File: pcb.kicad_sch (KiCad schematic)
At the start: 16 parts, among them IC1 BQ25606RGER, J1 PTHF-126-02-GF-Q-368, J1 Screw_Terminal_01x05, J2 Screw_Terminal_01x05, J3 Conn_01x01_Male

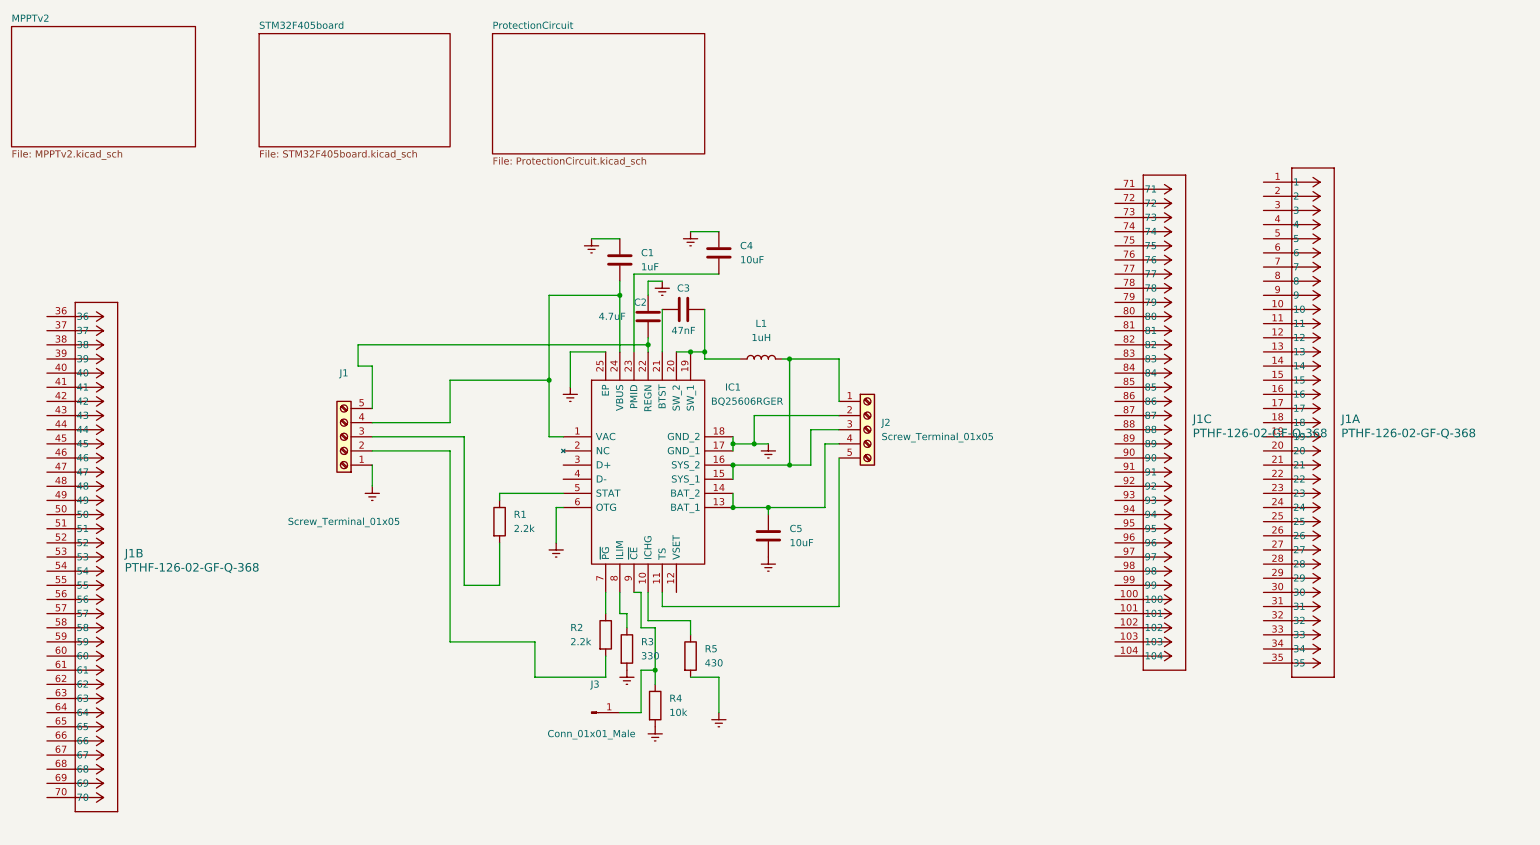
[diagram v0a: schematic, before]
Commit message: Major
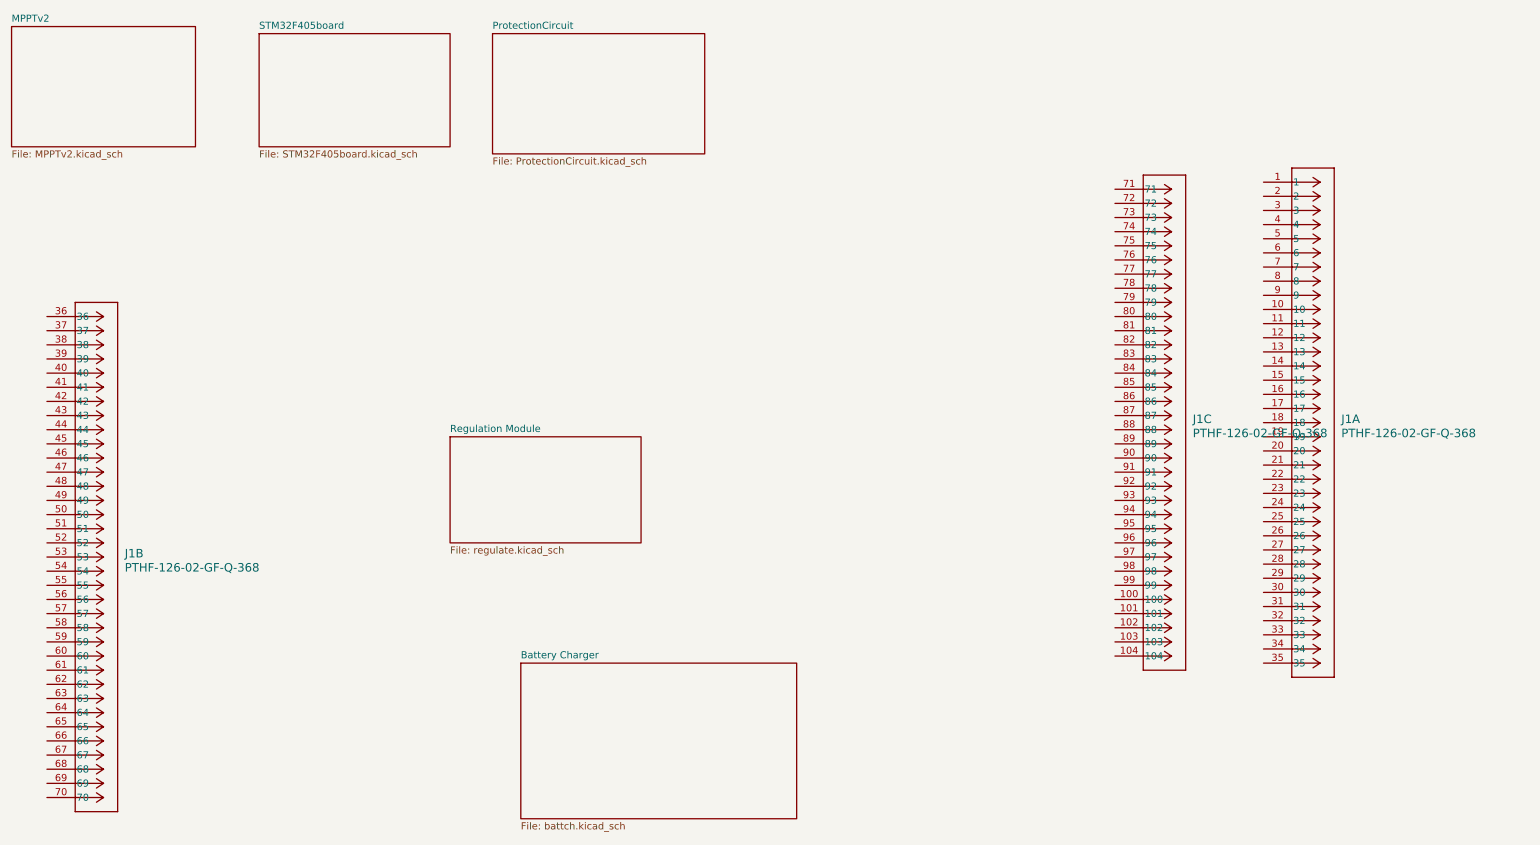
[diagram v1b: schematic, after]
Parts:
- removed C1: 1uF, 1uF cap:C1206, symbol Device:C
- removed C2: 4.7uF, cap 4.7uf:C1210, symbol Device:C
- removed C3: 47nF, 47nF:C1005_Commercial, symbol Device:C
- removed C4, C5: 10uF, 10uF MLCC:CAPC2012X94N, symbol Device:C
- removed IC1: BQ25606RGER, QFN50P400X400X100-25N-D, symbol BQ25606RGER:BQ25606RGER
- removed J1, J2: Screw_Terminal_01x05, TerminalBlock_MetzConnect:TerminalBlock_MetzConnect_Type059_RT06305HBWC_1x05_P3.50mm_Horizontal, symbol Connector:Screw_Terminal_01x05
- removed J3: Conn_01x01_Male, Connector_PinHeader_1.00mm:PinHeader_1x01_P1.00mm_Vertical, symbol Connector:Conn_01x01_Male
- removed L1: 1uH, 1uH indc:IHHP0805ZHER1R0M01, symbol Device:L
- removed R1, R2: 2.2k, 2.2k rst:RESC2012X65N, symbol Device:R
- removed R3: 330, rst 330:H2C_H2R, symbol Device:R
- removed R4: 10k, 10k rst:ERA8KEB1004V, symbol Device:R
- removed R5: 430, rst 430:ERJH3, symbol Device:R
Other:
- added sheet Battery Charger (battch.kicad_sch)
- added sheet Regulation Module (regulate.kicad_sch)
